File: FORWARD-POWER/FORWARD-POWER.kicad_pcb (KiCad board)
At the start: 2 copper layers, 49.5 x 40 mm, 23 parts, among them J1 Conn_01x02_Pin, J2 Conn_01x03_Pin, SW1 SW_SP3T, U1 AMS1117-3.3, U2 TPS63070RNMR

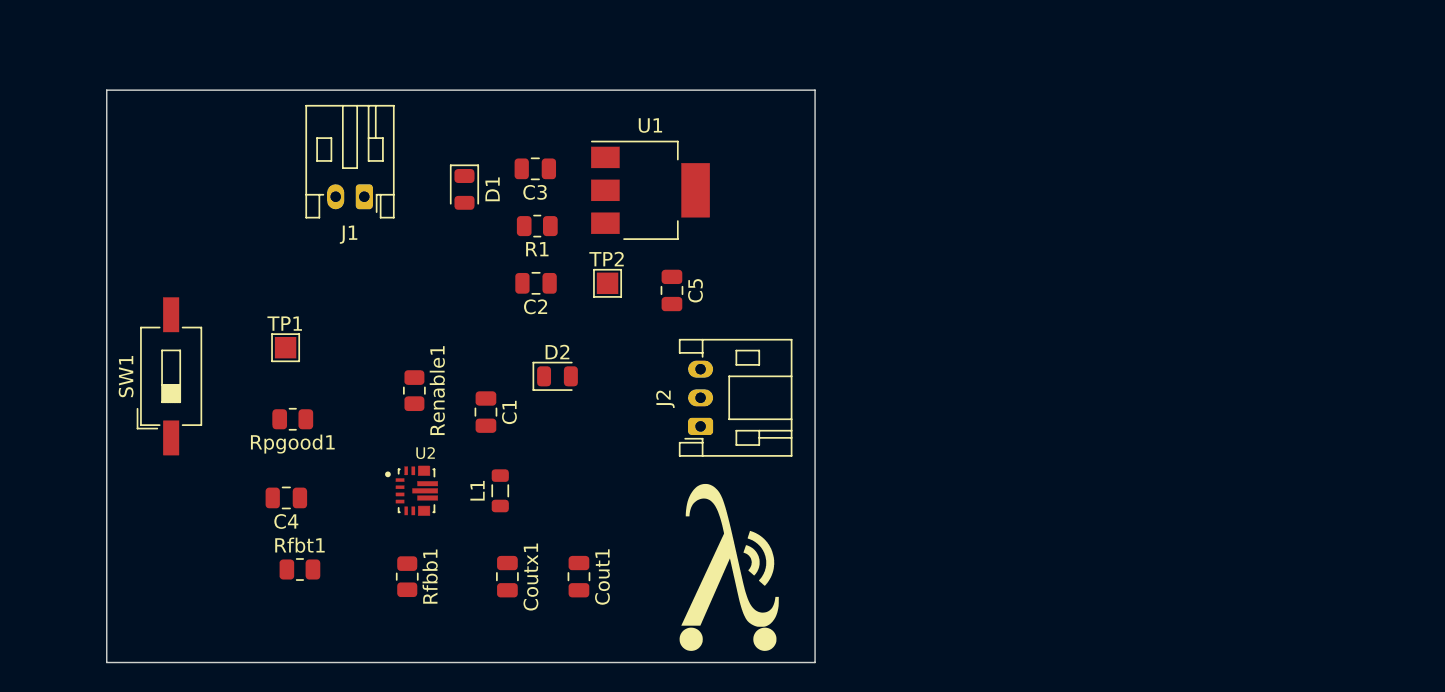
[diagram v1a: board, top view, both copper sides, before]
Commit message: itried
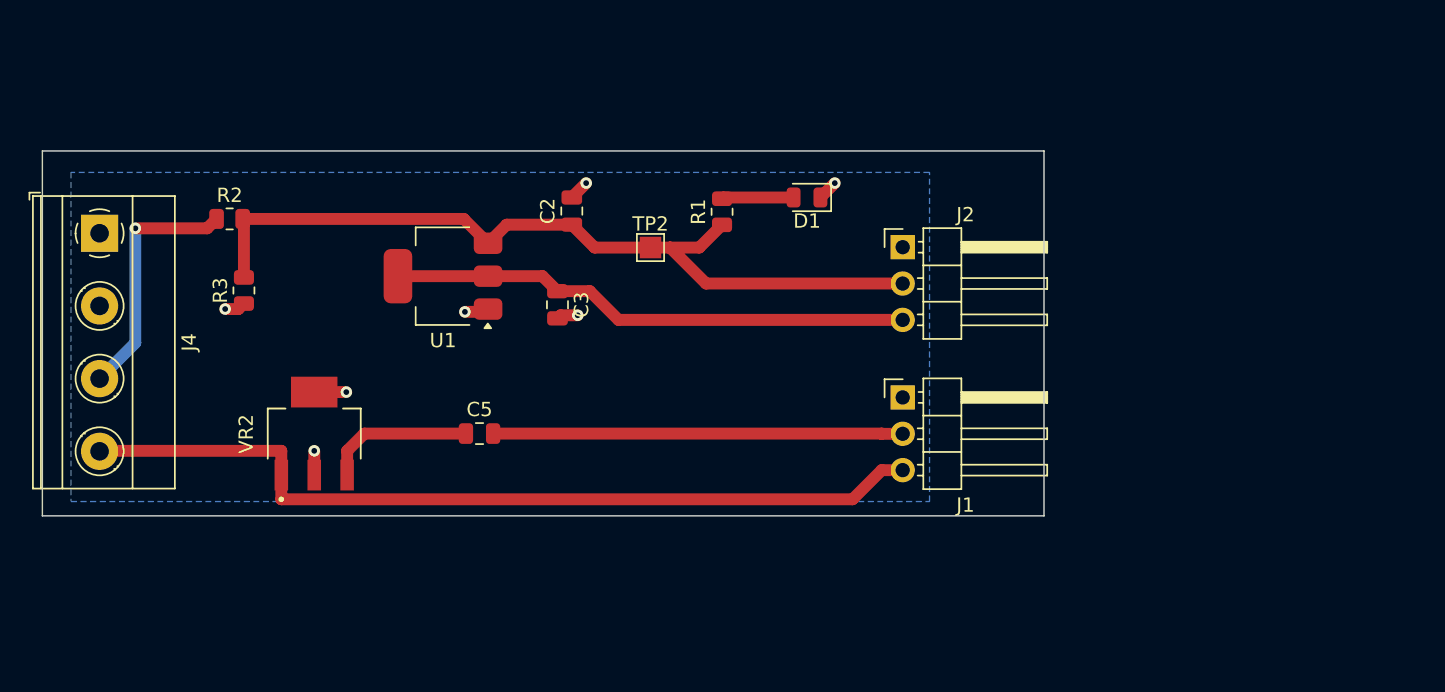
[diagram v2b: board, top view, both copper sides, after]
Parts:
- removed C1, Cout1: 47uF, Capacitor_SMD:C_0805_2012Metric
- removed C4: 100nF, Capacitor_SMD:C_0805_2012Metric
- removed Coutx1: 10uF, Capacitor_SMD:C_0805_2012Metric
- removed D2: LED, LED_SMD:LED_0805_2012Metric
- removed G***: LOGO, PCB design:lambda
- removed L1: 1.5uH, Inductor_SMD:L_0805_2012Metric
- removed Renable1: 10k, Resistor_SMD:R_0805_2012Metric
- removed Rfbb1, Rpgood1: 100k, Resistor_SMD:R_0805_2012Metric
- removed Rfbt1: 523k, Resistor_SMD:R_0805_2012Metric
- removed SW1: SW_SP3T, Button_Switch_SMD:SW_DIP_SPSTx01_Slide_6.7x4.1mm_W8.61mm_P2.54mm_LowProfile
- removed TP1: TestPoint, TestPoint:TestPoint_Pad_1.5x1.5mm
- removed U2: TPS63070RNMR, pcb-footprints:VREG_TPS63070RNMR
- added J4: Screw_Terminal_01x04, TerminalBlock_Phoenix:TerminalBlock_Phoenix_MKDS-1,5-4-5.08_1x04_P5.08mm_Horizontal, F.Cu at (158.5, 102.0)
- added R2: 1k, Resistor_SMD:R_0805_2012Metric, F.Cu at (167.6, 101.0)
- added R3: 5k, Resistor_SMD:R_0805_2012Metric, F.Cu at (168.6, 106.0)
- added VR2: LM7805MPX_NOPB, footprints:VREG_LM7805MPX_NOPB, F.Cu at (173.5, 116.0)
- C5: value 100nF -> 220uF
- J1: value Conn_01x02_Pin -> Conn_01x03_Pin; footprint Connector_JST:JST_PH_S2B-PH-K_1x02_P2.00mm_Horizontal -> Connector_PinHeader_2.54mm:PinHeader_1x03_P2.54mm_Horizontal
- J2: footprint Connector_JST:JST_PH_S3B-PH-K_1x03_P2.00mm_Horizontal -> Connector_PinHeader_2.54mm:PinHeader_1x03_P2.54mm_Horizontal
- moved J1 40.2 mm to (214.6, 113.5), turned to 0 degrees
- moved D1 23.9 mm to (207.9, 99.5), turned to 180 degrees
- moved J2 18.9 mm to (214.6, 103.0), turned to 0 degrees
- moved C5 16.8 mm to (185.1, 116.0), turned to 0 degrees
- moved U1 15.7 mm to (182.5, 105.0), turned to 180 degrees
- moved R1 13.0 mm to (202.0, 100.5), turned to 90 degrees
- moved C3 9.63 mm to (190.5, 107.0), turned to -90 degrees
- moved C2 5.63 mm to (191.5, 100.5), turned to 90 degrees
- moved TP2 3.91 mm to (197.0, 103.0)
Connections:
- C2 pad 1: +5V -> /anet
- C5 pad 1: +3.3V -> Net-(VR2-OUTPUT)
- C5 pad 2: GND -> +5V
- J1 pad 1: +6V -> GND
- J1 pad 2: GND -> +5V
- J2 pad 2: +5V -> /anet
- R1 pad 1: +5V -> /anet
- TP2 pad 1: +5V -> /anet
- U1 pad 3: +5V -> /anet
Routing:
- net +12V: track 0.00 -> 60.4 mm
- net /anet: track 0.00 -> 57.5 mm
- net +3.3V: track 0.00 -> 36.5 mm
- net +5V: track 0.00 -> 28.6 mm
- net +6V: track 0.00 -> 17.5 mm, vias 0 -> 1
- net GND: track 0.00 -> 11.4 mm, vias 0 -> 7
- net Net-(VR2-OUTPUT): track 0.00 -> 10.5 mm
- net Net-(D1-A): track 0.00 -> 5.04 mm
- added copper zone on B.Cu, net GND
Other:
- board size 49.5 x 40 mm -> 70 x 25.5 mm

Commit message: regulator pcb done
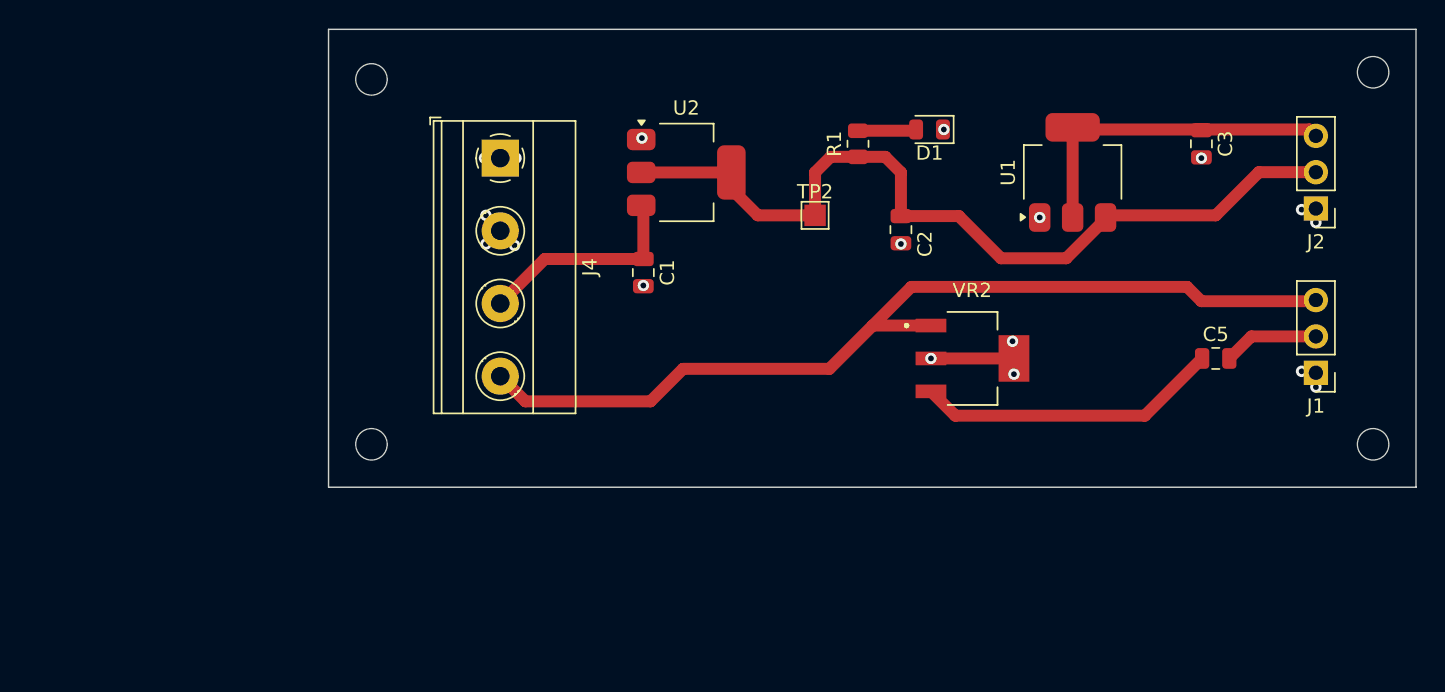
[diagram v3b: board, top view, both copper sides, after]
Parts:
- removed R2: 1k, Resistor_SMD:R_0805_2012Metric
- removed R3: 5k, Resistor_SMD:R_0805_2012Metric
- added C1: 47uF, Capacitor_SMD:C_0805_2012Metric, F.Cu at (196.5, 104.8)
- added H1: MountingHole, MountingHole:MountingHole_2.2mm_M2, F.Cu at (177.5, 91.2)
- added H2: MountingHole, MountingHole:MountingHole_2.2mm_M2, F.Cu at (177.5, 116.8)
- added H3: MountingHole, MountingHole:MountingHole_2.2mm_M2, F.Cu at (247.5, 90.8)
- added H4: MountingHole, MountingHole:MountingHole_2.2mm_M2, F.Cu at (247.5, 116.8)
- added U2: AMS1117-5.0, Package_TO_SOT_SMD:SOT-223-3_TabPin2, F.Cu at (199.5, 97.8)
- J1, J2: footprint Connector_PinHeader_2.54mm:PinHeader_1x03_P2.54mm_Horizontal -> Connector_PinHeader_2.54mm:PinHeader_1x03_P2.54mm_Vertical
- moved C5 51.7 mm to (236.5, 110.8)
- moved C3 46.4 mm to (235.5, 95.8)
- moved VR2 46.3 mm to (219.5, 110.8), turned to 0 degrees
- moved U1 44.6 mm to (226.5, 97.8), turned to 90 degrees
- moved J2 29.0 mm to (243.5, 100.3), turned to 180 degrees
- moved J1 28.9 mm to (243.5, 111.8), turned to 180 degrees
- moved J4 28.5 mm to (186.5, 96.8)
- moved C2 23.0 mm to (214.5, 101.8), turned to -90 degrees
- moved TP2 11.7 mm to (208.5, 100.8)
- moved R1 10.6 mm to (211.5, 95.8)
- moved D1 9.79 mm to (216.5, 94.8)
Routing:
- net +5V: track 28.6 -> 6.69 mm
- net +3.3V: track 36.5 -> 23.6 mm
- net Net-(VR2-OUTPUT): track 10.5 -> 21.3 mm
- net GND: track 11.4 -> 5.80 mm, vias 7 -> 18
- net +12V: track 60.4 -> 65.6 mm
- net /anet: track 57.5 -> 59.8 mm
- net +6V: track 17.5 -> 15.3 mm, vias 1 -> 0
- net Net-(D1-A): track 5.04 -> 4.10 mm
- added copper zone on In1.Cu, net GND
- removed copper zone on B.Cu, net GND
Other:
- board size 70 x 25.5 mm -> 76 x 32 mm
- copper layers 2 -> 4
